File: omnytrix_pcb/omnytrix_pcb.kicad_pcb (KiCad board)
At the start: 2 copper layers, 38 x 45.5 mm, 25 parts, among them J1 Conn_01x07, J2 Micro_SD_Card_Det2, SW1 SW_Push, U1 LD3985M33R_SOT23, U3 STM32F411RCTx

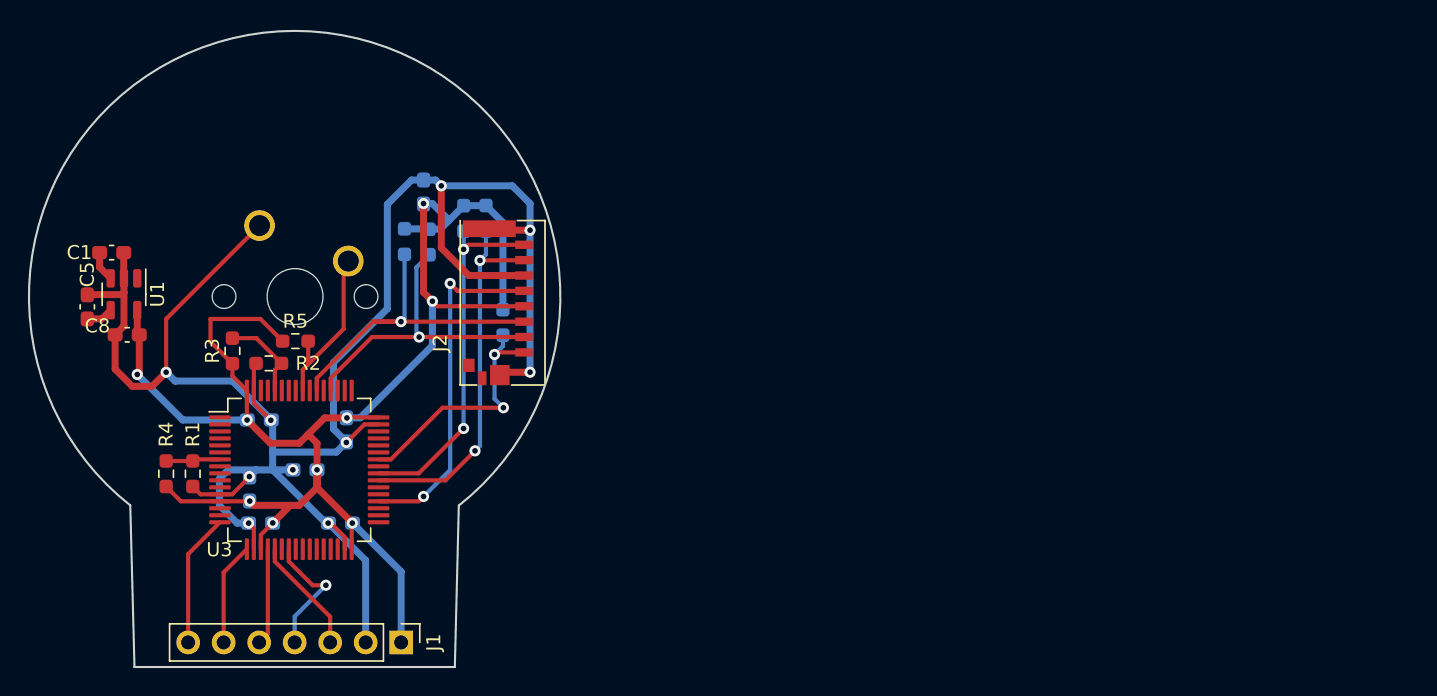
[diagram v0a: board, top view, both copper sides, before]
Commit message: compare topor and my trace
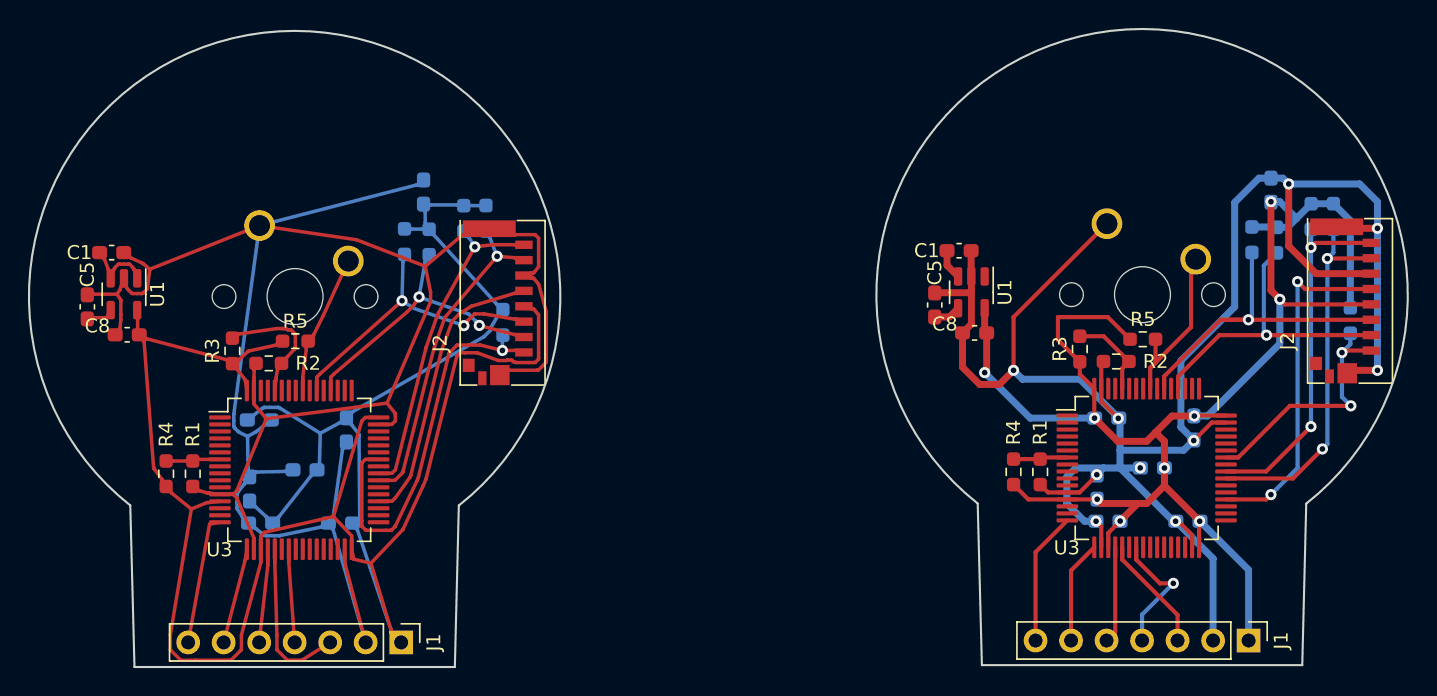
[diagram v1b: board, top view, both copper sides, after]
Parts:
- added C1: 1mkF, Capacitor_SMD:C_0603_1608Metric_Pad1.08x0.95mm_HandSolder, F.Cu at (147.5, 96.7)
- added C10: 100nF, Capacitor_SMD:C_0603_1608Metric_Pad1.08x0.95mm_HandSolder, B.Cu at (169.8, 92.4)
- added C2: 10mkF, Capacitor_SMD:C_0603_1608Metric_Pad1.08x0.95mm_HandSolder, B.Cu at (161.4, 112.3)
- added C3: 100nF, Capacitor_SMD:C_0603_1608Metric_Pad1.08x0.95mm_HandSolder, B.Cu at (158.1, 108.7)
- added C4: 100nF, Capacitor_SMD:C_0603_1608Metric_Pad1.08x0.95mm_HandSolder, B.Cu at (164.3, 109.4)
- added C5: byp10nF, Capacitor_SMD:C_0603_1608Metric_Pad1.08x0.95mm_HandSolder, F.Cu at (145.8, 100.6)
- added C6: 100nF, Capacitor_SMD:C_0603_1608Metric_Pad1.08x0.95mm_HandSolder, B.Cu at (163.9, 116.1)
- added C7: 100nF, Capacitor_SMD:C_0603_1608Metric_Pad1.08x0.95mm_HandSolder, B.Cu at (157.4, 113.6)
- added C8: 1mkF, Capacitor_SMD:C_0603_1608Metric_Pad1.08x0.95mm_HandSolder, F.Cu at (148.6, 102.6)
- added C9: 100nF, Capacitor_SMD:C_0603_1608Metric_Pad1.08x0.95mm_HandSolder, B.Cu at (158.2, 116.1)
- added J1: Conn_01x07, Connector_PinHeader_2.54mm:PinHeader_1x07_P2.54mm_Vertical, F.Cu at (168.2, 124.6)
- added J2: Micro_SD_Card_Det2, libs:microSD_molex, F.Cu at (178.7, 94.3)
- added R1: 100k, Resistor_SMD:R_0603_1608Metric_Pad0.98x0.95mm_HandSolder, F.Cu at (153.3, 112.5)
- added R10: 47k, Resistor_SMD:R_0603_1608Metric_Pad0.98x0.95mm_HandSolder, B.Cu at (168.5, 95.9)
- added R2: 100k, Resistor_SMD:R_0603_1608Metric_Pad0.98x0.95mm_HandSolder, F.Cu at (158.8, 104.6)
- added R3: 10k, Resistor_SMD:R_0603_1608Metric_Pad0.98x0.95mm_HandSolder, F.Cu at (156.2, 103.7)
- added R4: 10k, Resistor_SMD:R_0603_1608Metric_Pad0.98x0.95mm_HandSolder, F.Cu at (151.4, 112.5)
- added R5: 10k, Resistor_SMD:R_0603_1608Metric_Pad0.98x0.95mm_HandSolder, F.Cu at (160.7, 103.1)
- added R6: 47k, Resistor_SMD:R_0603_1608Metric_Pad0.98x0.95mm_HandSolder, B.Cu at (172.7, 94.3)
- added R7: 47k, Resistor_SMD:R_0603_1608Metric_Pad0.98x0.95mm_HandSolder, B.Cu at (174.3, 94.3)
- added R8: 47k, Resistor_SMD:R_0603_1608Metric_Pad0.98x0.95mm_HandSolder, B.Cu at (170.2, 96.0)
- added R9: 47k, Resistor_SMD:R_0603_1608Metric_Pad0.98x0.95mm_HandSolder, B.Cu at (175.5, 101.7)
- added SW1: SW_Push, Button_Switch_Keyboard:SW_Cherry_MX_1.00u_PCB, B.Cu at (158.1, 94.8)
- added U1: LD3985M33R_SOT23, Package_TO_SOT_SMD:SOT-23-5, F.Cu at (148.4, 99.7)
- added U3: STM32F411RCTx, Package_QFP:LQFP-64_10x10mm_P0.5mm, F.Cu at (161.0, 112.3)
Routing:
- net +3.3V: track 118.2 -> 290.6 mm
- net GND: track 149.0 -> 314.0 mm
- net /SD_D2: track 18.3 -> 46.6 mm, vias 2 -> 3
- net /SD_D1: track 26.0 -> 49.2 mm, vias 2 -> 3
- net /SD_D0: track 27.0 -> 50.1 mm, vias 2 -> 3
- net /SD_CMD: track 24.3 -> 46.3 mm, vias 1 -> 3
- net /SD_D3: track 22.3 -> 43.1 mm, vias 1 -> 3
- net /SD_CK: track 24.9 -> 45.2 mm
- net /SCL: track 8.31 -> 20.0 mm
- net /BTN: track 12.9 -> 22.9 mm
- net /RST: track 9.54 -> 18.9 mm
- net BOOT0: track 6.40 -> 15.7 mm
- net /CS: track 7.36 -> 14.2 mm
- net /DC: track 6.93 -> 13.6 mm
- net /SDA: track 9.25 -> 15.9 mm
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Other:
- board size 38 x 45.5 mm -> 98.6 x 45.6 mm
